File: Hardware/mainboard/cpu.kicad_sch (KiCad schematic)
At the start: 27 parts, among them J301 Conn_02x05_Odd_Even, SW102 DNP, U301 MIMXRT1176DVMAA, Y301 24MHz, Y302 32.768K

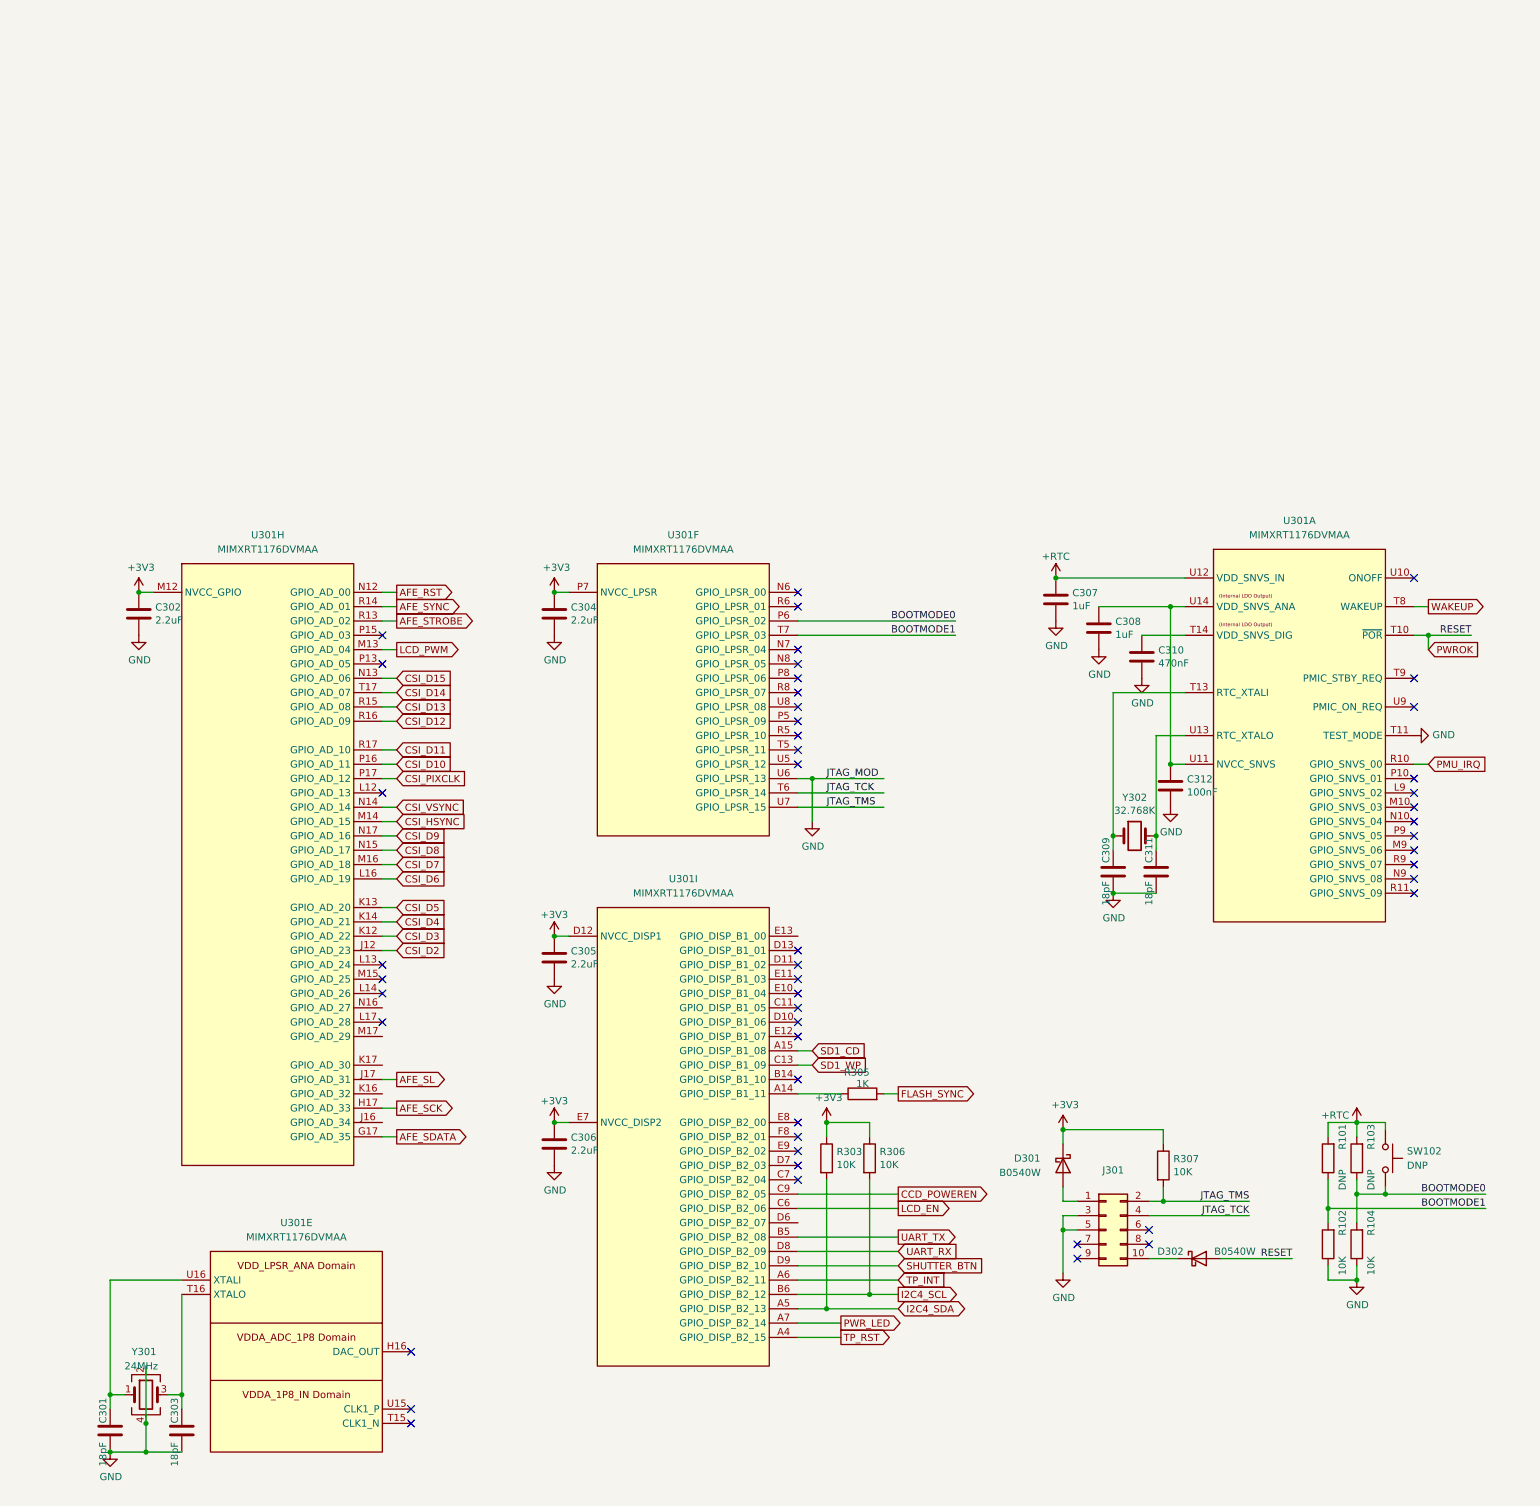
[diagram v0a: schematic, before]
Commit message: New mainboard rev wip
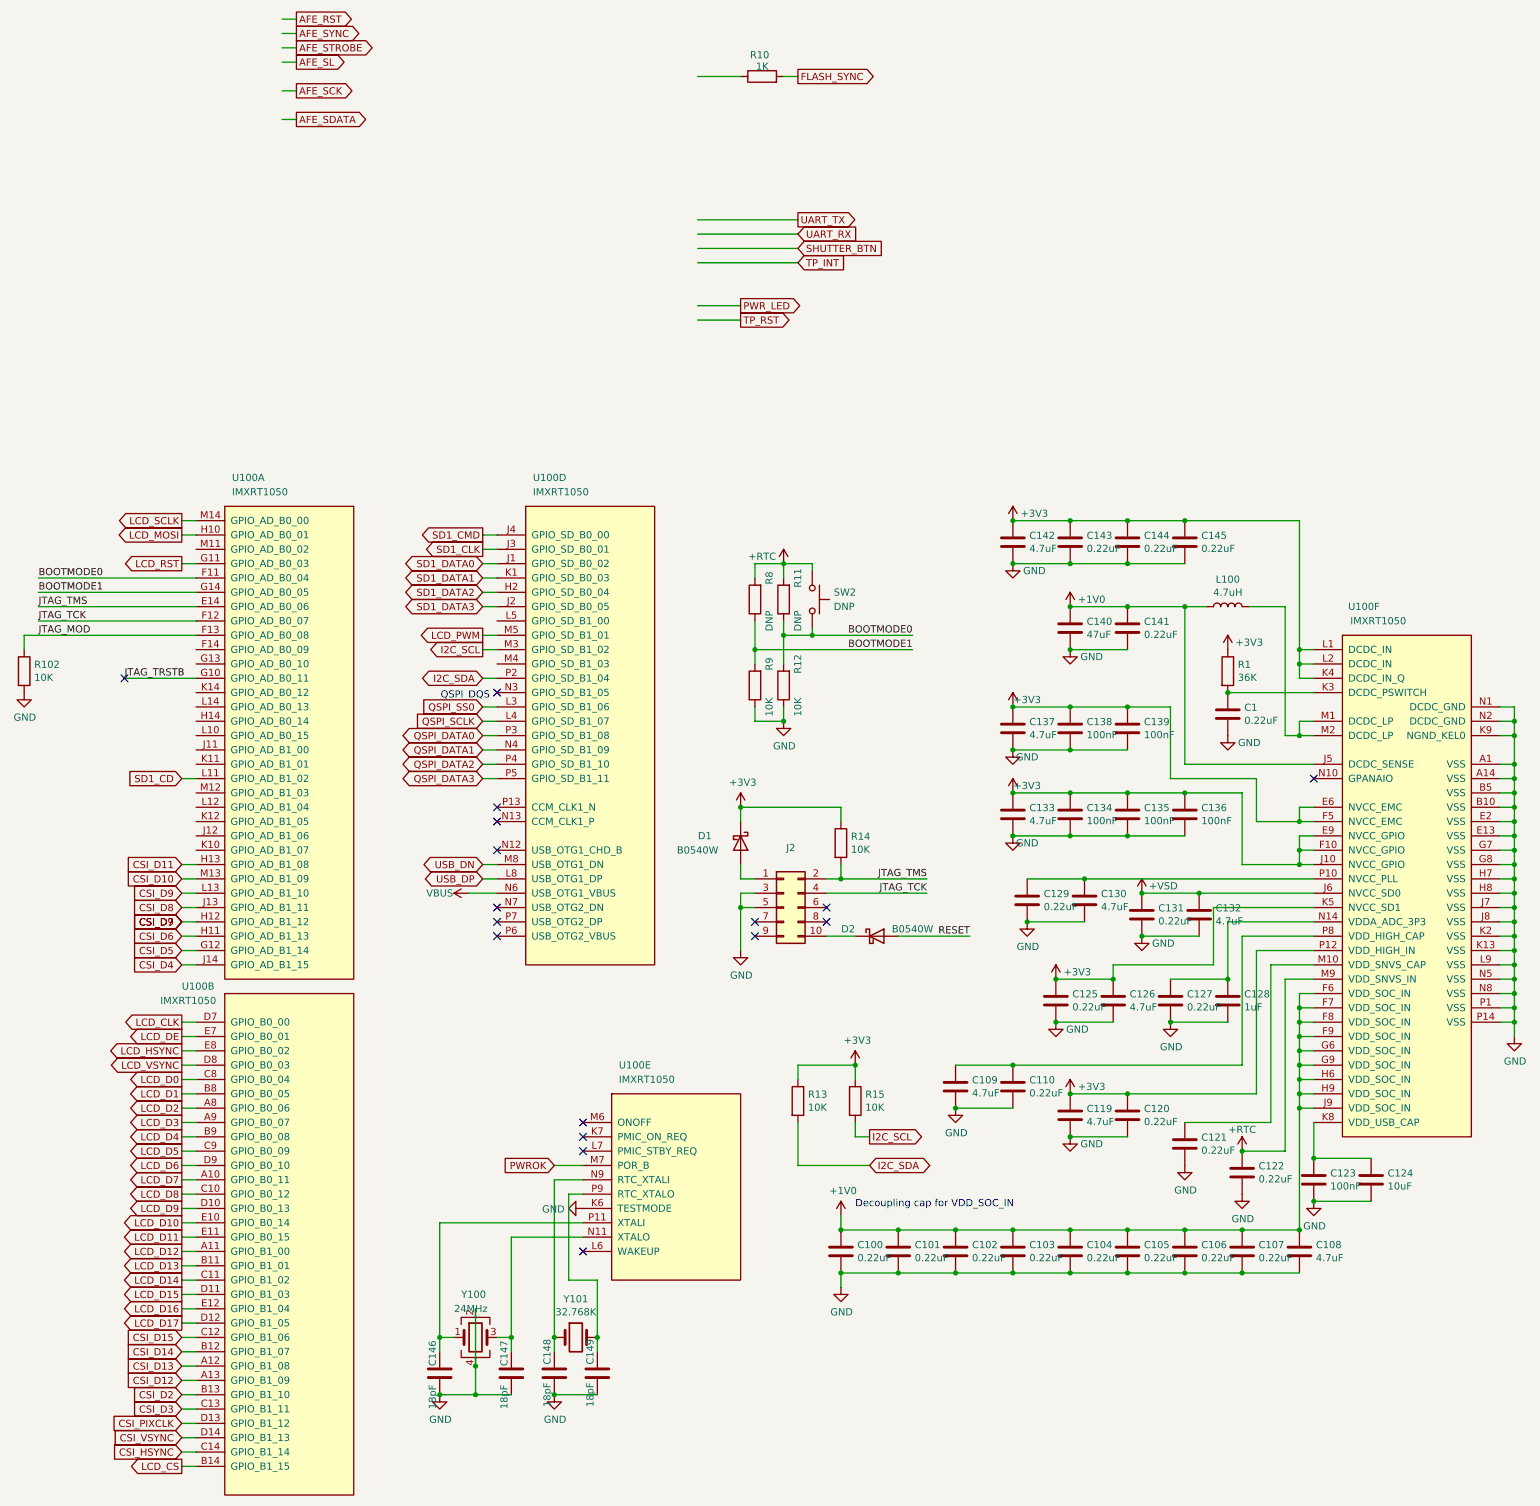
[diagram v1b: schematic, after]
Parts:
- removed C301, C303, C309, C311: 18pF, Capacitor_SMD:C_0402_1005Metric, symbol Device:C
- removed C302, C304, C305, C306: 2.2uF, Capacitor_SMD:C_0402_1005Metric, symbol Device:C
- removed C307, C308: 1uF, Capacitor_SMD:C_0402_1005Metric, symbol Device:C
- removed C310: 470nF, Capacitor_SMD:C_0402_1005Metric, symbol Device:C
- removed C312: 100nF, Capacitor_SMD:C_0402_1005Metric, symbol Device:C
- removed R303, R306: 10K, Resistor_SMD:R_0402_1005Metric, symbol Device:R
- removed U301: MIMXRT1176DVMAA, footprints:BGA-289_17x17_14.0x14.0mm, symbol symbols:MIMXRT1176DVMAA
- removed Y301: 24MHz, Oscillator:Oscillator_SMD_Abracon_ASE-4Pin_3.2x2.5mm, symbol Device:Crystal_GND24
- removed Y302: 32.768K, Crystal:Crystal_SMD_TXC_9HT11-2Pin_2.0x1.2mm_HandSoldering, symbol Device:Crystal
- added C1, C100, C101, C102, C103, C104, C105, C106, C107, C110, C120, C121, C122, C125, C127, C129, C131, C141, C143, C144, C145: 0.22uF, Capacitor_SMD:C_0402_1005Metric, symbol Device:C
- added C108, C109, C119, C126, C130, C132, C133, C137, C142: 4.7uF, Capacitor_SMD:C_0603_1608Metric, symbol Device:C
- added C123, C134, C135, C136, C138, C139: 100nF, Capacitor_SMD:C_0402_1005Metric, symbol Device:C
- added C124: 10uF, Capacitor_SMD:C_0603_1608Metric, symbol Device:C
- added C128: 1uF, Capacitor_SMD:C_0402_1005Metric, symbol Device:C
- added C140: 47uF, Capacitor_SMD:C_0603_1608Metric, symbol Device:C
- added C146, C147, C148, C149: 18pF, Capacitor_SMD:C_0402_1005Metric, symbol Device:C
- added L100: 4.7uH, Inductor_SMD:L_Vishay_IHLP-1212, symbol Device:L
- added R1: 36K, Resistor_SMD:R_0402_1005Metric, symbol Device:R
- added R102, R13, R15: 10K, Resistor_SMD:R_0402_1005Metric, symbol Device:R
- added U100: IMXRT1050, footprints:BGA-196_14x14_12.0x12.0mm, symbol Sitina:IMXRT1050
- added Y100: 24MHz, Oscillator:Oscillator_SMD_Abracon_ASE-4Pin_3.2x2.5mm, symbol Device:Crystal_GND24
- added Y101: 32.768K, Crystal:Crystal_SMD_TXC_9HT11-2Pin_2.0x1.2mm_HandSoldering, symbol Device:Crystal
- renumbered D301 to D1, D302 to D2, J301 to J2, R305 to R10, R103 to R11, R104 to R12, R307 to R14, R101 to R8, R102 to R9, SW102 to SW2
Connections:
- net +3V3: now also C119.1, C120.1, C125.1, C126.1, C133.1, C134.1, C135.1, C136.1, C137.1, C138.1, C139.1, C142.1, C143.1, C144.1, C145.1, R1.1, R13.1, R15.1, U100.E6 (NVCC_EMC), U100.E9 (NVCC_GPIO), U100.F10 (NVCC_GPIO), U100.F5 (NVCC_EMC), U100.J10 (NVCC_GPIO), U100.K4 (DCDC_IN_Q), U100.K5 (NVCC_SD1), U100.L1 (DCDC_IN), U100.L2 (DCDC_IN), U100.P12 (VDD_HIGH_IN)
- net +RTC: now also C122.1, U100.M9 (VDD_SNVS_IN)
- net BOOTMODE0: now also U100.F11 (GPIO_AD_B0_04)
- net BOOTMODE1: now also U100.G14 (GPIO_AD_B0_05)
- net CSI_D10: now also U100.M13 (GPIO_AD_B1_09)
- net CSI_D11: now also U100.H13 (GPIO_AD_B1_08)
- net CSI_D12: now also U100.A13 (GPIO_B1_09)
- net CSI_D13: now also U100.A12 (GPIO_B1_08)
- net CSI_D14: now also U100.B12 (GPIO_B1_07)
- net CSI_D15: now also U100.C12 (GPIO_B1_06)
- net CSI_D2: now also U100.B13 (GPIO_B1_10)
- net CSI_D3: now also U100.C13 (GPIO_B1_11)
- net CSI_D4: now also U100.J14 (GPIO_AD_B1_15)
- net CSI_D5: now also U100.G12 (GPIO_AD_B1_14)
- net CSI_D6: now also U100.H11 (GPIO_AD_B1_13)
- net CSI_D7: now also U100.H12 (GPIO_AD_B1_12), U100.L13 (GPIO_AD_B1_10)
- net CSI_D8: now also U100.J13 (GPIO_AD_B1_11)
- net CSI_HSYNC: now also U100.C14 (GPIO_B1_14)
- net CSI_PIXCLK: now also U100.D13 (GPIO_B1_12)
- net CSI_VSYNC: now also U100.D14 (GPIO_B1_13)
- net GND: now also C1.2, C100.2, C101.2, C102.2, C103.2, C104.2, C105.2, C106.2, C107.2, C108.2, C109.2, C110.2, C119.2, C120.2, C121.2, C122.2, C123.2, C124.2, C125.2, C126.2, C127.2, C128.2, C129.2, C130.2, C131.2, C132.2, C133.2, C134.2, C135.2, C136.2, C137.2, C138.2, C139.2, C140.2, C141.2, C142.2, C143.2, C144.2, C145.2, C146.2, C147.2, C148.1, C149.1, R102.2, U100.A1 (VSS), U100.A14 (VSS), U100.B10 (VSS), U100.B5 (VSS), U100.E13 (VSS), U100.E2 (VSS), U100.G7 (VSS), U100.G8 (VSS), U100.H7 (VSS), U100.H8 (VSS), U100.J7 (VSS), U100.J8 (VSS), U100.K13 (VSS), U100.K2 (VSS), U100.K6 (TESTMODE), U100.K9 (NGND_KEL0), U100.L9 (VSS), U100.N1 (DCDC_GND), U100.N2 (DCDC_GND), U100.N5 (VSS), U100.N8 (VSS), U100.P1 (VSS), U100.P14 (VSS), Y100.2, Y100.4
- net JTAG_TCK: now also U100.F12 (GPIO_AD_B0_07)
- net JTAG_TMS: now also U100.E14 (GPIO_AD_B0_06)
- net LCD_PWM: now also U100.M5 (GPIO_SD_B1_01)
- net PWROK: now also U100.M7 (POR_B); no longer D2.2 (A)
- net SD1_CD: now also U100.L11 (GPIO_AD_B1_02)
- new net: C129.1, C130.1, U100.P10 (NVCC_PLL)
- new net: C1.1, R1.2, U100.K3 (DCDC_PSWITCH)
- new net: C123.1, C124.1, U100.K8 (VDD_USB_CAP)
- new net: L100.2, U100.M1 (DCDC_LP), U100.M2 (DCDC_LP)
- new net: C121.1, U100.M10 (VDD_SNVS_CAP)
- new net: C127.1, C128.1, U100.N14 (VDDA_ADC_3P3)
- new net: C109.1, C110.1, U100.P8 (VDD_HIGH_CAP)
- new net: C147.1, U100.N11 (XTALO), Y100.3
- new net: C149.2, U100.P9 (RTC_XTALO), Y101.2
- new net: C148.2, U100.N9 (RTC_XTALI), Y101.1
- new net: C146.1, U100.P11 (XTALI), Y100.1
- new net +1V0: C100.1, C101.1, C102.1, C103.1, C104.1, C105.1, C106.1, C107.1, C108.1, C140.1, C141.1, L100.1, U100.F6 (VDD_SOC_IN), U100.F7 (VDD_SOC_IN), U100.F8 (VDD_SOC_IN), U100.F9 (VDD_SOC_IN), U100.G6 (VDD_SOC_IN), U100.G9 (VDD_SOC_IN), U100.H6 (VDD_SOC_IN), U100.H9 (VDD_SOC_IN), U100.J5 (DCDC_SENSE), U100.J9 (VDD_SOC_IN)
- new net +VSD: C131.1, C132.1, U100.J6 (NVCC_SD0)
- new net I2C_SCL: R15.2, U100.M3 (GPIO_SD_B1_02)
- new net I2C_SDA: R13.2, U100.P2 (GPIO_SD_B1_04)
- new net JTAG_MOD: R102.1, U100.F13 (GPIO_AD_B0_08)
- new net JTAG_TRSTB: U100.G10 (GPIO_AD_B0_11)
- new net LCD_CLK: U100.D7 (GPIO_B0_00)
- new net LCD_CS: U100.B14 (GPIO_B1_15)
- new net LCD_D0: U100.C8 (GPIO_B0_04)
- new net LCD_D1: U100.B8 (GPIO_B0_05)
- new net LCD_D10: U100.E10 (GPIO_B0_14)
- new net LCD_D11: U100.E11 (GPIO_B0_15)
- new net LCD_D12: U100.A11 (GPIO_B1_00)
- new net LCD_D13: U100.B11 (GPIO_B1_01)
- new net LCD_D14: U100.C11 (GPIO_B1_02)
- new net LCD_D15: U100.D11 (GPIO_B1_03)
- new net LCD_D16: U100.E12 (GPIO_B1_04)
- new net LCD_D17: U100.D12 (GPIO_B1_05)
- new net LCD_D2: U100.A8 (GPIO_B0_06)
- new net LCD_D3: U100.A9 (GPIO_B0_07)
- new net LCD_D4: U100.B9 (GPIO_B0_08)
- new net LCD_D5: U100.C9 (GPIO_B0_09)
- new net LCD_D6: U100.D9 (GPIO_B0_10)
- new net LCD_D7: U100.A10 (GPIO_B0_11)
- new net LCD_D8: U100.C10 (GPIO_B0_12)
- new net LCD_D9: U100.D10 (GPIO_B0_13)
- new net LCD_DE: U100.E7 (GPIO_B0_01)
- new net LCD_HSYNC: U100.E8 (GPIO_B0_02)
- new net LCD_MOSI: U100.H10 (GPIO_AD_B0_01)
- new net LCD_RST: U100.G11 (GPIO_AD_B0_03)
- new net LCD_SCLK: U100.M14 (GPIO_AD_B0_00)
- new net LCD_VSYNC: U100.D8 (GPIO_B0_03)
- new net QSPI_DATA0: U100.P3 (GPIO_SD_B1_08)
- new net QSPI_DATA1: U100.N4 (GPIO_SD_B1_09)
- new net QSPI_DATA2: U100.P4 (GPIO_SD_B1_10)
- new net QSPI_DATA3: U100.P5 (GPIO_SD_B1_11)
- new net QSPI_SCLK: U100.L4 (GPIO_SD_B1_07)
- new net QSPI_SS0: U100.L3 (GPIO_SD_B1_06)
- new net RESET: D2.2 (A)
- new net SD1_CLK: U100.J3 (GPIO_SD_B0_01)
- new net SD1_CMD: U100.J4 (GPIO_SD_B0_00)
- new net SD1_DATA0: U100.J1 (GPIO_SD_B0_02)
- new net SD1_DATA1: U100.K1 (GPIO_SD_B0_03)
- new net SD1_DATA2: U100.H2 (GPIO_SD_B0_04)
- new net SD1_DATA3: U100.J2 (GPIO_SD_B0_05)
- new net USB_DN: U100.M8 (USB_OTG1_DN)
- new net USB_DP: U100.L8 (USB_OTG1_DP)
- new net VBUS: U100.N6 (USB_OTG1_VBUS)
- no-connect marks 50 -> 17
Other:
- note added: "Decoupling cap for VDD_SOC_IN"
- note added: "QSPI_DQS"
- moved on the sheet: D1, D2, J2, R10, R11, R12, R14, R8, R9, SW2
